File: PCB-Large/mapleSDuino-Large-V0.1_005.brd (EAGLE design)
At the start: 79 x 27 mm, 24 parts, among them IC2 LAN-USR-ES1

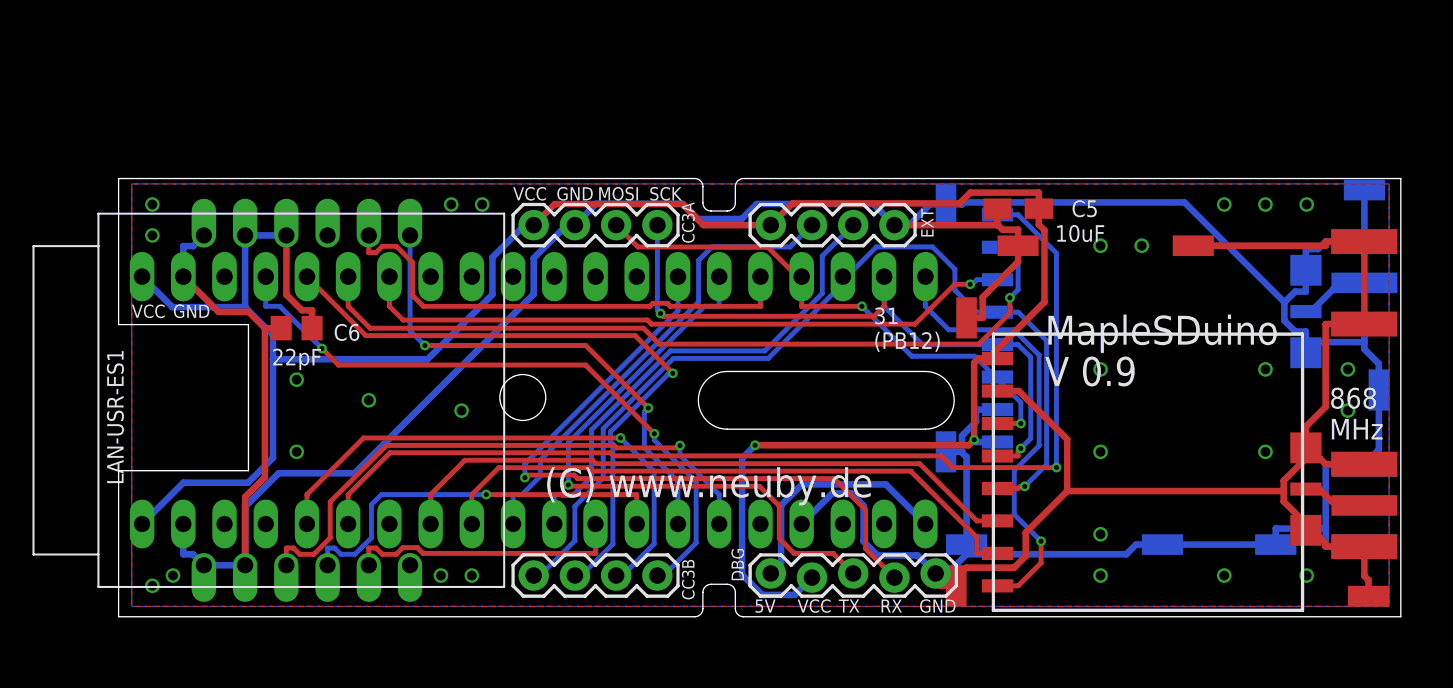
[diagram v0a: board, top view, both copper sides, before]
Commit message: Large 1st try; v009 Schematic
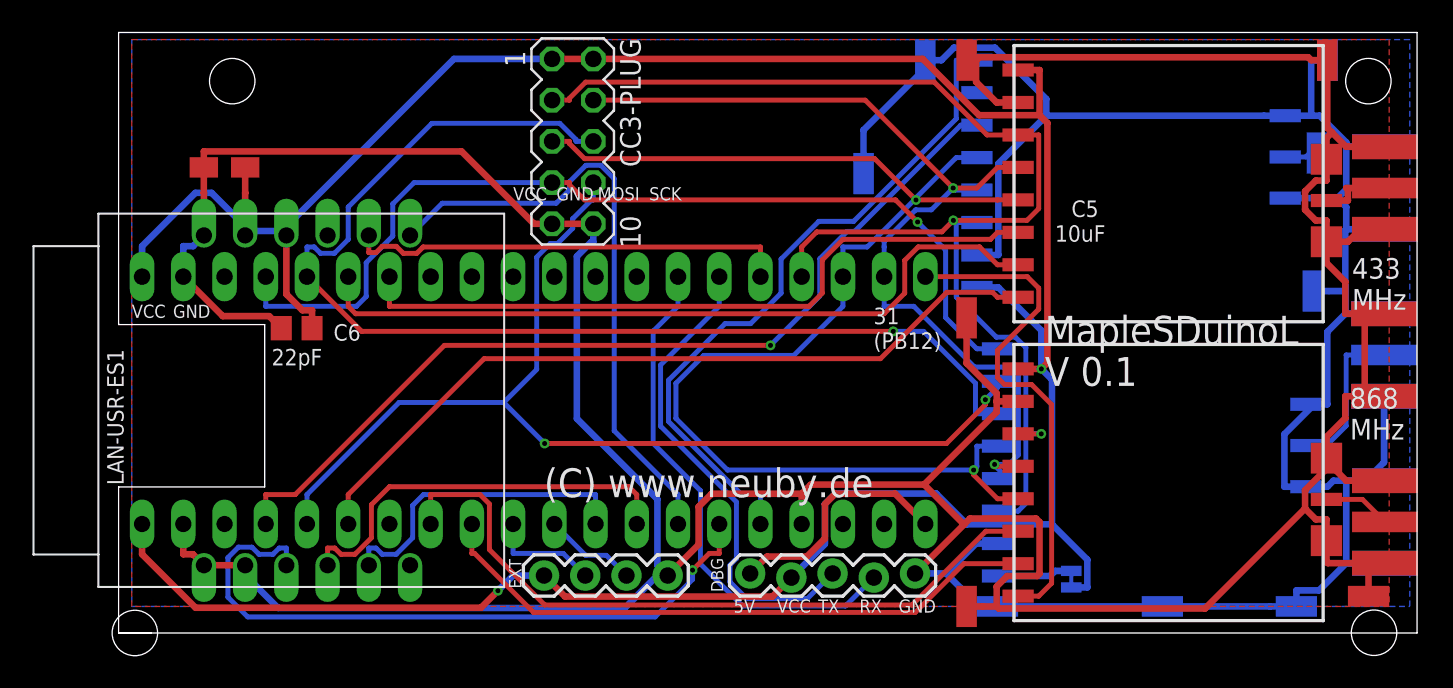
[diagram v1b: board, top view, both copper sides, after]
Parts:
- removed CC0: CC1101, CC1101:CC1101_MODULE1_SMD
- removed CC3A, CC3B: (no value), SparkFun-Connectors:1X04
- added CC2: CC1101_MODULE1SMD, CC1101:CC1101_MODULE1_SMD
- added CC3, CC4: CC1101_MODULE1SMD, wireless:CC1101_MODULE1_SMD
- added CC3-PLUG: (no value), con-lstb:MA05-2
- added PAD13: WIREPADSMD1,27-254, wirepad:SMD1,27-2,54
- added VTRX2: JUMPER-SMT_2_NC_TRACE_SILK, SparkFun-Jumpers:SMT-JUMPER_2_NC_TRACE_SILK
- added X3: (no value), adafruit:SMA_EDGELAUNCH
- CC1: value CC1101_MODULE1SMD -> CC1101
- moved C5 49.0 mm to (9.53, 27.7)
- moved EXT 25.7 mm to (29.2, 2.54)
- moved PAD11 23.7 mm to (48.9, 27.3), turned to 180 degrees
- moved CC1 23.5 mm to (58.4, 1.27), flipped to the top, turned to 0 degrees
- moved PAD10 20.6 mm to (77.5, 34.3)
- moved PAD5 14.1 mm to (77.5, 34.3), turned to 180 degrees
- moved PAD3 11.9 mm to (55.2, 34.3), turned to 180 degrees
- moved PAD8 10.0 mm to (57.1, 0.64), turned to 270 degrees
- moved PAD12 8.98 mm to (52.7, 34.3)
- moved PAD9 6.99 mm to (76.6, 20.1), turned to 180 degrees
- moved X2 5.98 mm to (83.1, 26.4), flipped to the top, turned to 180 degrees
- moved PAD4 4.02 mm to (75.6, 0.64)
- moved PAD7 3.81 mm to (67.3, 0.64)
- moved X1 1.63 mm to (83.1, 5.84)
- moved PAD6 1.42 mm to (55.2, 0.64)
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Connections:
- new net ANT3: CC3.ANT, X3.P
- new net CC_OUT_3: CC4.GDO0
- new net N$1: CC3.VCC, VTRX2.2
- new net N$2: CC4.ANT, PAD13.1
- net ANT1: now also CC2.ANT; no longer CC1.ANT
- net ANT2: now also CC1.ANT; no longer CC0.ANT
- net CC_CS0: now also CC1.CSN; no longer CC0.CSN
- net CC_CS1: now also CC2.CSN; no longer CC1.CSN
- net CC_CS2: now also CC3-PLUG.7, CC3.CSN; no longer CC3B.4
- net CC_CS3: now also CC4.CSN
- net CC_IN_0: now also CC1.GDO2; no longer CC0.GDO2
- net CC_IN_1: now also CC2.GDO2; no longer CC1.GDO2
- net CC_IN_2: now also CC3-PLUG.6, CC3.GDO2; no longer CC3B.2
- net CC_IN_3: now also CC4.GDO2
- net CC_OUT_0: now also CC1.GDO0; no longer CC0.GDO0
- net CC_OUT_1: now also CC2.GDO0; no longer CC1.GDO0
- net CC_OUT_2: now also CC3-PLUG.8, CC3.GDO0; no longer CC3B.3
- net GND: now also CC2.GND@0, CC2.GND@1, CC2.GND@2, CC3-PLUG.10, CC3-PLUG.9, CC3.GND@0, CC3.GND@1, CC3.GND@2, CC4.GND@0, CC4.GND@1, CC4.GND@2, X3.GND@1, X3.GND@2, X3.GND@3, X3.GND@4; no longer CC0.GND@0, CC0.GND@1, CC0.GND@2, CC3A.2
- net MISO2: now also CC2.MISO, CC3-PLUG.5, CC3.MISO, CC4.MISO; no longer CC0.MISO, CC3B.1
- net MOSI2: now also CC2.MOSI, CC3-PLUG.3, CC3.MOSI, CC4.MOSI; no longer CC0.MOSI, CC3A.3
- net SCK2: now also CC2.SCLK, CC3-PLUG.4, CC3.SCLK, CC4.SCLK; no longer CC0.SCLK, CC3A.4
- net VCC: now also CC2.VCC, CC3-PLUG.1, CC3-PLUG.2, CC4.VCC, VTRX2.1; no longer CC0.VCC, CC3A.1
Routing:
- net GND: track 295.3 -> 406.7 mm, vias 27 -> 0
- net CC_IN_3: track 0.00 -> 56.4 mm, vias 0 -> 1
- net VCC: track 141.3 -> 187.2 mm
- net MOSI2: track 33.5 -> 79.4 mm
- net CC_CS3: track 0.00 -> 42.4 mm
- net CC_OUT_2: track 33.1 -> 65.9 mm, vias 1 -> 2
- net CC_IN_2: track 40.5 -> 71.7 mm
- net MISO2: track 57.8 -> 85.1 mm, vias 1 -> 2
- net RX2: track 30.2 -> 5.76 mm
- net TX2: track 29.2 -> 6.82 mm
- net CC_CS2: track 40.0 -> 59.2 mm, vias 2 -> 1
- net SCK2: track 41.3 -> 60.2 mm
- net CC_CS1: track 64.7 -> 48.4 mm, vias 1 -> 0
- net RX1: track 43.1 -> 32.0 mm, vias 1 -> 0
- net ANT3: track 0.00 -> 9.69 mm
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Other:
- board size 79 x 27 mm -> 80 x 37 mm
- board text added: "MapleSDuinoL"
- board text added: "MapleSDuinoL V0.1"
- board text added: "V 0.1"
- board text removed: "CS2"
- board text removed: "IN2"
- board text removed: "MISO2"
- board text removed: "MapleSDuino"
- board text removed: "MapleSDuino V0.9"
- board text removed: "OUT2"
- board text removed: "V 0.9"
